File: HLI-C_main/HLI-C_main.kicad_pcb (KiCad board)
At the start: 2 copper layers, 27.9 x 55 mm, 59 parts, among them CON1 USB_B, CON3 CR123A, CON4 Conn_02x05_Odd_Even, Q1 IRLML5103, U1 PIC24HJ64GP206-I_PT, U2 FM25V10-GTR, U3 FT232RL, U5 TPS7A0533PDBV, U6 LM3658SD, U7 TPS7A0533PDBV, U8 ATSHA204A-SSHDA-B, U9 24AA02-OT, Y1 Crystal_32KHz, Y2 Crystal_20MHz

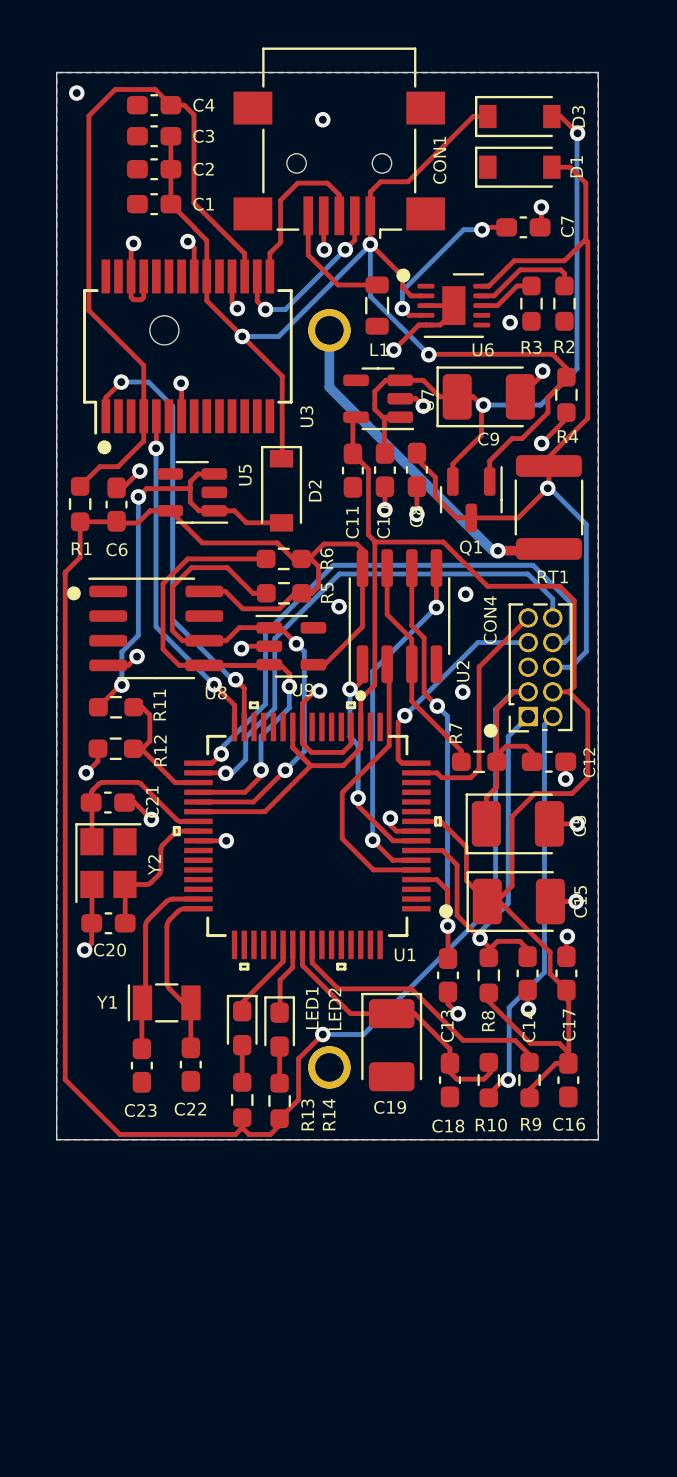
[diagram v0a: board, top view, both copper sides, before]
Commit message: att
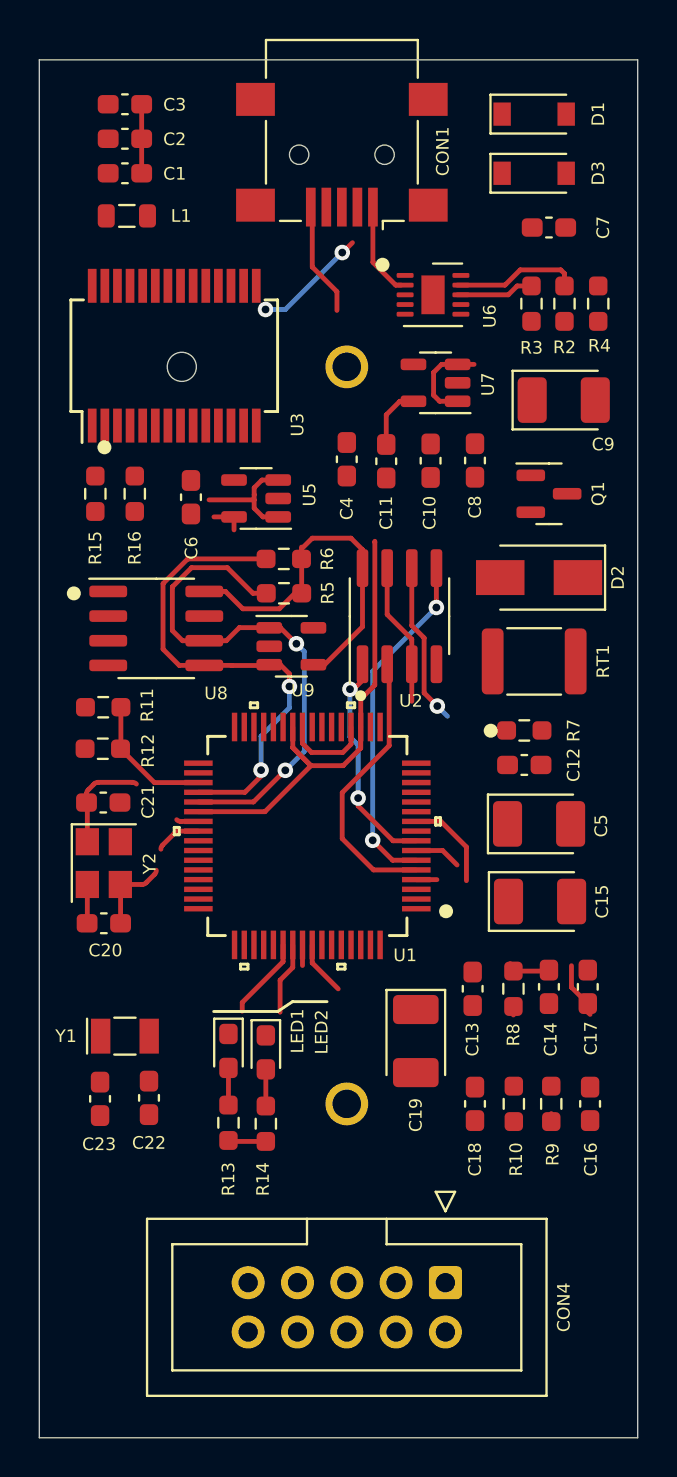
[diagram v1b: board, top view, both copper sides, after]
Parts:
- removed R1: 0R, Resistor_SMD:R_0603_1608Metric_Pad0.98x0.95mm_HandSolder
- added R15: 470R, Resistor_SMD:R_0603_1608Metric_Pad0.98x0.95mm_HandSolder, F.Cu at (179.8, 40.9)
- added R16: 470R, Resistor_SMD:R_0603_1608Metric_Pad0.98x0.95mm_HandSolder, F.Cu at (181.9, 40.9)
- C11: value 100nF -> 1uF
- C20, C21: value 10pF -> 20pF
- C22, C23: value 7pF -> 12pF
- CON4: value Conn_02x05_Odd_Even -> Conector_gravação; footprint Connector_PinSocket_1.27mm:PinSocket_2x05_P1.27mm_Vertical -> Connector_IDC:IDC-Header_2x05_P2.54mm_Vertical
- D1, D3: value SSA33L -> DSS14U
- D2: value SSA33L -> S1D-13F; footprint Diode_SMD:D_SOD-123 -> Diode_SMD:D_SMA
- moved CON4 29.5 mm to (197.9, 81.5), turned to -90 degrees
- moved C4 20.8 mm to (192.8, 39.1), turned to -90 degrees
- moved D2 14.0 mm to (202.7, 45.2), turned to 180 degrees
- moved L1 13.7 mm to (181.5, 26.6), turned to 0 degrees
- moved RT1 7.97 mm to (202.4, 49.5), turned to 180 degrees
- moved R4 4.98 mm to (205.7, 31.1)
- moved Q1 4.01 mm to (203.2, 40.9), turned to 0 degrees
- moved C9 3.87 mm to (204.0, 36.1)
- moved C6 3.85 mm to (184.8, 41.1)
- moved U5 3.30 mm to (188.1, 41.1)
- moved U7 3.07 mm to (197.4, 35.2)
- moved C8 3.03 mm to (199.4, 39.2)
- moved D3 3.02 mm to (202.4, 24.4)
- moved R7 2.83 mm to (201.9, 53.1)
- moved D1 2.83 mm to (202.4, 21.3)
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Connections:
- CON3 pad N: 0 -> (no net)
- D1 pad 1: 0 -> +5V
- D1 pad 2: VBAT -> +5VD
- D2 pad 1: +5V -> 0
- D2 pad 2: +5VD -> VBAT
- D3 pad 2: Net-(C10-Pad1) -> unconnected-(D3-Pad2)
- U1 pad 11: K0 -> unconnected-(U1-Pad11)
- U1 pad 12: K1 -> unconnected-(U1-Pad12)
- U1 pad 13: K2 -> unconnected-(U1-Pad13)
- U1 pad 14: K3 -> unconnected-(U1-Pad14)
- U1 pad 18: KC -> unconnected-(U1-Pad18)
- U1 pad 21: KD -> unconnected-(U1-Pad21)
- U1 pad 22: KE -> unconnected-(U1-Pad22)
- U1 pad 23: K4 -> unconnected-(U1-Pad23)
- U1 pad 24: K5 -> unconnected-(U1-Pad24)
- U1 pad 27: K6 -> unconnected-(U1-Pad27)
- U1 pad 28: K7 -> unconnected-(U1-Pad28)
- U1 pad 29: K8 -> unconnected-(U1-Pad29)
- U1 pad 30: K9 -> unconnected-(U1-Pad30)
- U1 pad 33: RXB -> unconnected-(U1-Pad33)
- U1 pad 34: TXB -> unconnected-(U1-Pad34)
- U1 pad 52: KB -> unconnected-(U1-Pad52)
- U1 pad 53: KA -> unconnected-(U1-Pad53)
- U3 pad 1: TXA -> Net-(U3-Pad1)
- U3 pad 5: RXA -> Net-(U3-Pad5)
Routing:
- net +3V3: track 116.5 -> 22.4 mm, vias 1 -> 0
- net +5V: track 64.4 -> 8.29 mm, vias 3 -> 0
- net +3.3VP: track 89.6 -> 35.9 mm
- net 0: track 56.0 -> 6.59 mm, vias 33 -> 0
- net VBAT: track 45.9 -> 0.00 mm, vias 1 -> 0
- net Net-(C4-Pad1): track 38.1 -> 0.00 mm
- net Net-(C10-Pad1): track 34.7 -> 4.46 mm, vias 2 -> 0
- net RXB: track 29.3 -> 0.00 mm, vias 1 -> 0
- net TXB: track 27.3 -> 0.00 mm, vias 1 -> 0
- net TXA: track 23.8 -> 0.00 mm, vias 2 -> 0
- net +2V5: track 21.1 -> 0.00 mm, vias 1 -> 0
- net RESET: track 23.4 -> 4.75 mm, vias 1 -> 0
- net RXA: track 18.0 -> 0.00 mm, vias 2 -> 0
- net Net-(CON3-Pad1): track 17.8 -> 0.00 mm, vias 1 -> 0
- net +5VD: track 22.4 -> 6.20 mm, vias 2 -> 0
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- removed copper zone on B.Cu, net 0
- removed copper zone on F.Cu, net 0
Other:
- board size 27.9 x 55 mm -> 30.8 x 71 mm
